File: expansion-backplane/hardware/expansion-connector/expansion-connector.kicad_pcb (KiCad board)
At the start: 2 copper layers, 39 x 45 mm, 2 parts

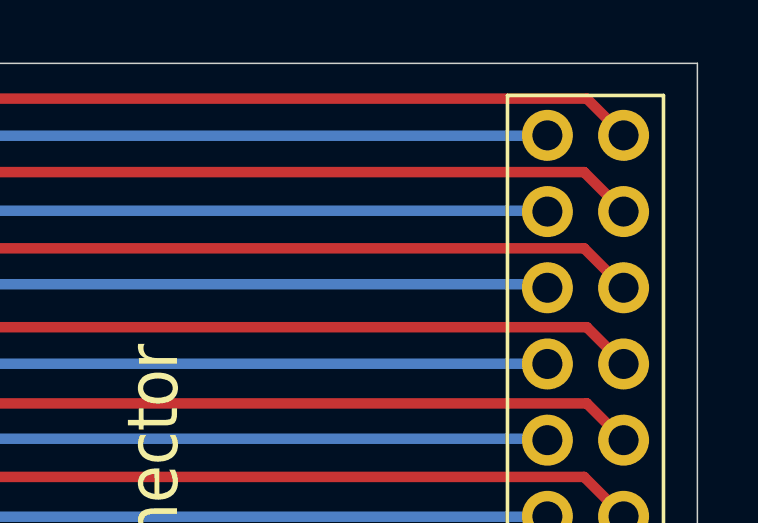
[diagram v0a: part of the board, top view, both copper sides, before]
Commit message: update speech pld file and more
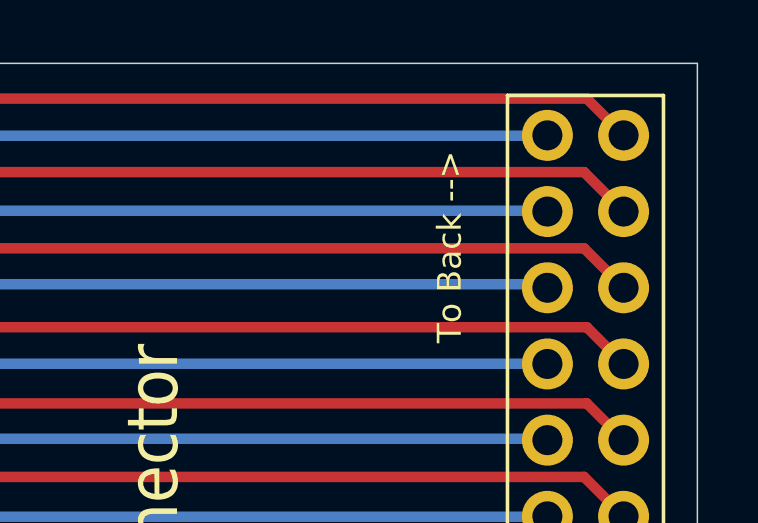
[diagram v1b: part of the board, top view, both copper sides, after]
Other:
- board text added: "To Back -->"
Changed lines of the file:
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@@
 			(outputformat 1)
 			(mirror no)
-			(drillshape 1)
+			(drillshape 0)
 			(scaleselection 1)
-			(outputdirectory "")
+			(outputdirectory "gerbers_v1")
 		)
 	)
@@
 		)
 	)
+	(gr_text "To Back -->"
+		(at 156.21 84.328 90)
+		(layer "F.SilkS")
+		(effects
+			(font
+				(size 0.8 0.8)
+				(thickness 0.1)
+			)
+			(justify left bottom)
+		)
+	)
